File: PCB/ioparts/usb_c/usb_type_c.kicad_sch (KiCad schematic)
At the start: 9 parts, among them J2 USB_C_Receptacle_USB2.0, J4 Conn_01x04

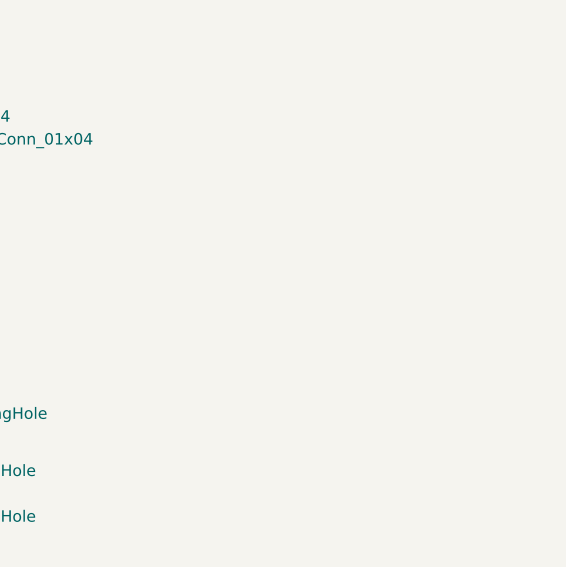
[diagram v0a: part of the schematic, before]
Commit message: misc pcbs
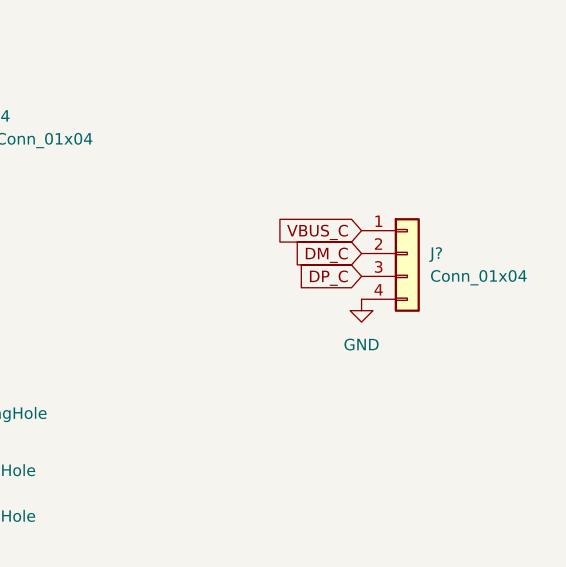
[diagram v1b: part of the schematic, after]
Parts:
- added J?: Conn_01x04, Connector_JST:JST_SH_SM04B-SRSS-TB_1x04-1MP_P1.00mm_Horizontal, symbol Connector_Generic:Conn_01x04
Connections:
- net DM_C: now also J?.2 (Pin_2)
- net DP_C: now also J?.3 (Pin_3)
- net GND: now also J?.4 (Pin_4)
- net VBUS_C: now also J?.1 (Pin_1)
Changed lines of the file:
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@@
     (stroke (width 0) (type default) (color 0 0 0 0))
+  )
+  (global_label "VBUS_C" (shape input) (at 166.37 74.93 180) (fields_autoplaced)
+    (effects (font (size 1.27 1.27)) (justify right))
+    (property "Intersheet References" "${INTERSHEET_REFS}" (id 0) (at 156.8207 74.8506 0)
+      (effects (font (size 1.27 1.27)) (justify right) hide)
+    )
   )
   (global_label "DP_C" (shape input) (at 91.44 62.23 0) (fields_autoplaced)
@@
     )
   )
+  (global_label "DM_C" (shape input) (at 166.37 77.47 180) (fields_autoplaced)
+    (effects (font (size 1.27 1.27)) (justify right))
+    (property "Intersheet References" "${INTERSHEET_REFS}" (id 0) (at 158.9979 77.3906 0)
+      (effects (font (size 1.27 1.27)) (justify right) hide)
+    )
+  )
   (global_label "SHIELD" (shape input) (at 66.04 95.25 270) (fields_autoplaced)
     (effects (font (size 1.27 1.27)) (justify right))
@@
     (effects (font (size 1.27 1.27)) (justify right))
     (property "Intersheet References" "${INTERSHEET_REFS}" (id 0) (at 68.5006 91.555 90)
+      (effects (font (size 1.27 1.27)) (justify right) hide)
+    )
+  )
+  (global_label "DP_C" (shape input) (at 166.37 80.01 180) (fields_autoplaced)
+    (effects (font (size 1.27 1.27)) (justify right))
+    (property "Intersheet References" "${INTERSHEET_REFS}" (id 0) (at 159.1793 79.9306 0)
       (effects (font (size 1.27 1.27)) (justify right) hide)
     )
@@
     (pin "1")
   )
+  (symbol (lib_id "Connector_Generic:Conn_01x04") (at 171.45 77.47 0) (unit 1)
+    (in_bom yes) (on_board yes) (fields_autoplaced)
+    (property "Reference" "J?" (id 0) (at 173.99 77.4699 0)
+      (effects (font (size 1.27 1.27)) (justify left))
+    )
+    (property "Value" "Conn_01x04" (id 1) (at 173.99 80.0099 0)
+      (effects (font (size 1.27 1.27)) (justify left))
+    )
+    (property "Footprint" "Connector_JST:JST_SH_SM04B-SRSS-TB_1x04-1MP_P1.00mm_Horizontal" (id 2) (at 171.45 77.47 0)
+      (effects (font (size 1.27 1.27)) hide)
+    )
+    (property "Datasheet" "~" (id 3) (at 171.45 77.47 0)
+      (effects (font (size 1.27 1.27)) hide)
+    )
+    (pin "1")
+    (pin "2")
+    (pin "3")
+    (pin "4")
+  )
+  (symbol (lib_id "power:GND") (at 166.37 82.55 0) (unit 1)
+    (in_bom yes) (on_board yes) (fields_autoplaced)
+    (property "Reference" "#PWR?" (id 0) (at 166.37 88.9 0)
+      (effects (font (size 1.27 1.27)) hide)
+    )
+    (property "Value" "GND" (id 1) (at 166.37 87.63 0))
+    (property "Footprint" "" (id 2) (at 166.37 82.55 0)
+      (effects (font (size 1.27 1.27)) hide)
+    )
+    (property "Datasheet" "" (id 3) (at 166.37 82.55 0)
+      (effects (font (size 1.27 1.27)) hide)
+    )
+    (pin "1")
+  )
   (symbol (lib_id "Device:R") (at 69.85 95.25 90) (unit 1)
     (in_bom yes) (on_board yes)
@@
       (reference "#PWR0105") (unit 1) (value "GND") (footprint "")
     )
+    (path "/ddf6b6a2-e871-407c-aeac-716dedc27429"
+      (reference "#PWR?") (unit 1) (value "GND") (footprint "")
+    )
     (path "/7670b80c-802b-43a2-92b4-83f5e059e974"
       (reference "H1") (unit 1) (value "MountingHole") (footprint "MountingHole:MountingHole_2.1mm")
@@
       (reference "J4") (unit 1) (value "Conn_01x04") (footprint "Connector_JST:JST_PH_S4B-PH-K_1x04_P2.00mm_Horizontal")
     )
+    (path "/b37be1a6-21b5-454f-a864-a94fa52c2591"
+      (reference "J?") (unit 1) (value "Conn_01x04") (footprint "Connector_JST:JST_SH_SM04B-SRSS-TB_1x04-1MP_P1.00mm_Horizontal")
+    )
     (path "/1f917771-93af-46ca-96b6-a65e04d7225f"
